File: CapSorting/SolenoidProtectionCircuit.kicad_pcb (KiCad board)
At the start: 2 copper layers, 30 x 30 mm, 15 parts, among them CN12 S6B-XH-A, Q1 2SA1015, Q12 2SA1015, Q13 IRLB8721PBF, Q2 IRLB8721PBF

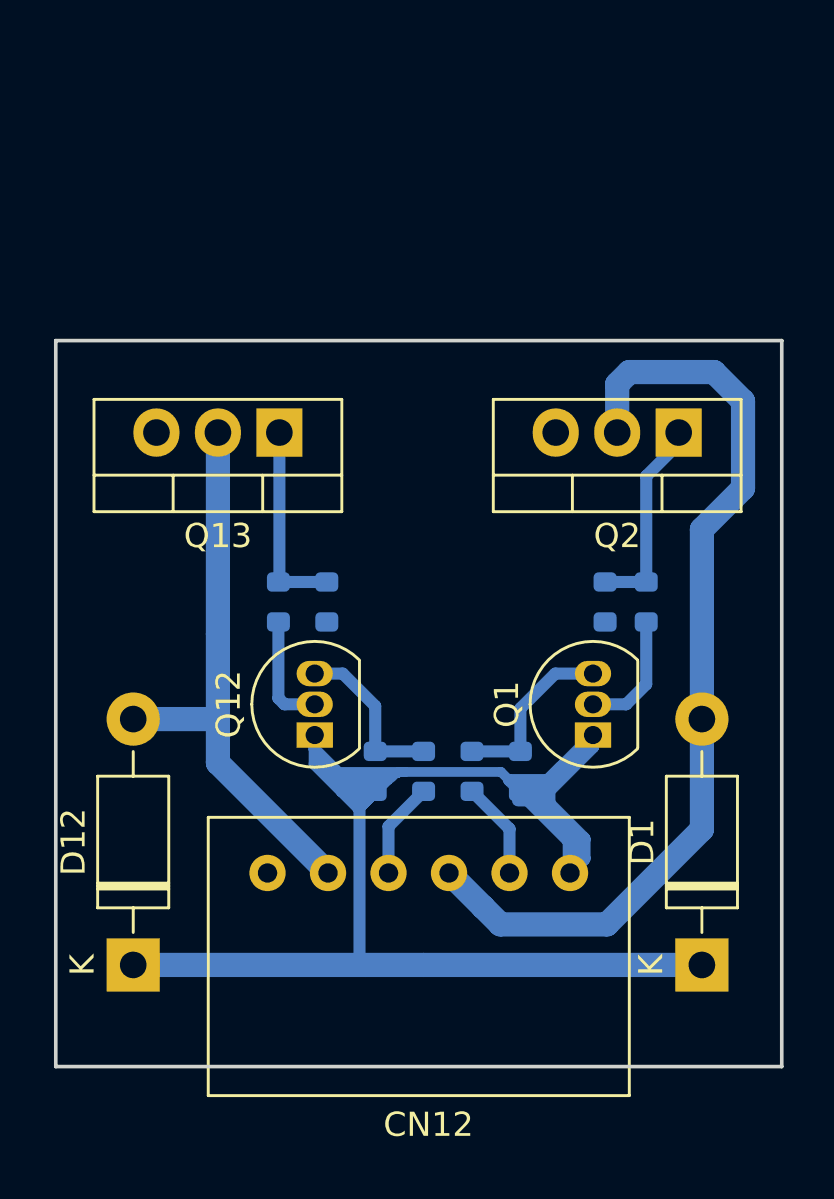
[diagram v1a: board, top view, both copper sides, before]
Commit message: 引き直し
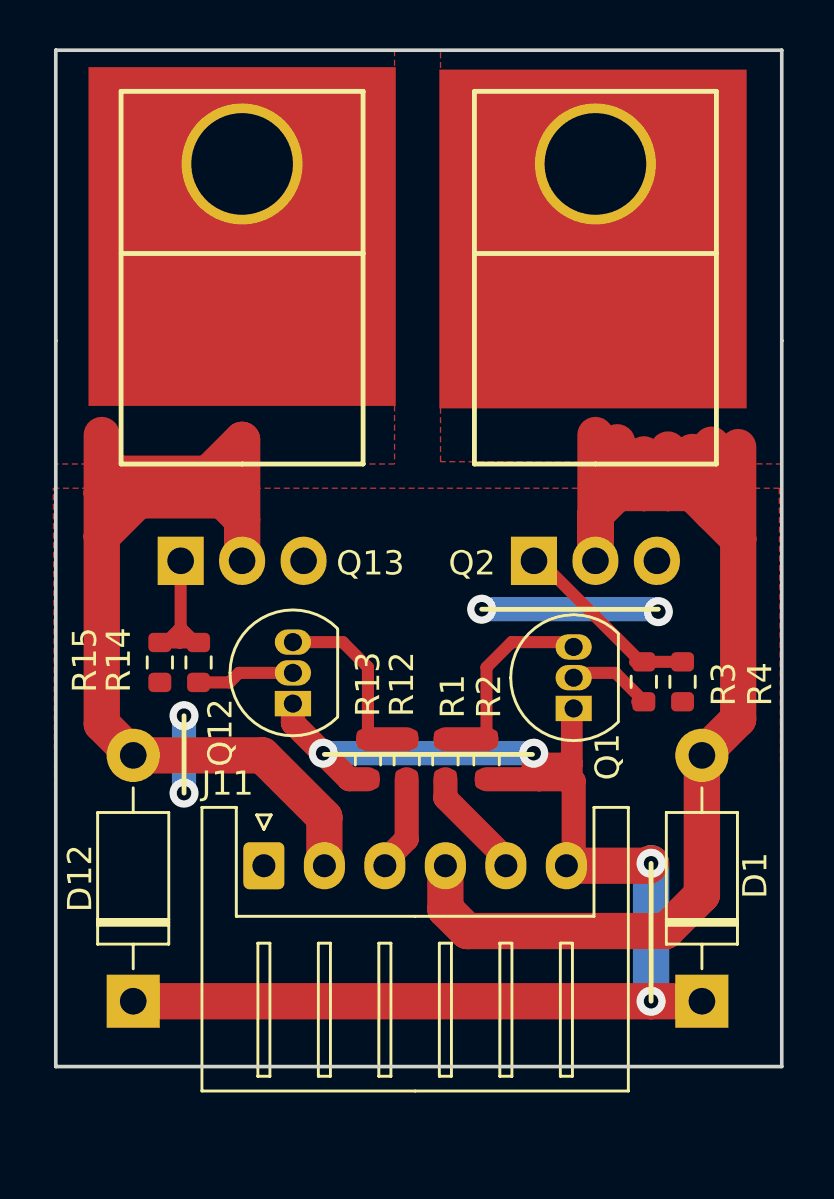
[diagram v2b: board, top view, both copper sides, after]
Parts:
- removed CN12: S6B-XH-A, JST:S6B-XH-A
- added J11: Conn_01x06, Connector_JST:JST_XH_S6B-XH-A_1x06_P2.50mm_Horizontal, F.Cu at (93.6, 99.7)
- Q13, Q2: footprint Package_TO_SOT_THT:TO-220-3_Vertical -> CapSorting:IRLB8721PBF-2
- R1, R12, R13, R14, R15, R2, R3, R4: moved to F.Cu
- moved R15 7.34 mm to (89.3, 91.3)
- moved Q2 6.32 mm to (107.3, 87.1), turned to 0 degrees
- moved Q13 5.52 mm to (92.7, 87.1), turned to 0 degrees
- moved R4 4.60 mm to (110.9, 92.1)
- moved R14 4.14 mm to (90.9, 91.3)
- moved R3 3.30 mm to (109.3, 92.1)
- moved Q12 1.58 mm to (94.8, 93.0)
- moved D1 1.50 mm to (111.7, 105.3)
- moved D12 1.50 mm to (88.2, 105.3)
- moved R2 1.49 mm to (102.8, 95.3)
- moved Q1 1.36 mm to (106.4, 93.2)
- moved R1 1.21 mm to (101.1, 95.3)
- moved R12 0.86 mm to (99.5, 95.3)
- moved R13 0.58 mm to (97.9, 95.3)
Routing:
- net Solenoid1: track 23.6 -> 43.2 mm
- net Solenoid2: track 39.3 -> 56.7 mm
- net +24V: track 74.0 -> 59.4 mm, vias 0 -> 4
- net GND: track 0.00 -> 10.5 mm, vias 0 -> 4
- net Net-(Q1-Pad2): track 5.12 -> 3.68 mm
- net Net-(Q1-Pad3): track 7.37 -> 8.71 mm
- net Net-(Q12-Pad3): track 6.93 -> 8.11 mm
- net Net-(Q13-Pad1): track 8.19 -> 7.10 mm
- net Net-(Q12-Pad2): track 4.76 -> 4.06 mm
- net PLC_Y012: track 4.02 -> 4.61 mm
- added copper zone on F.Cu, net GND
- added copper zone on F.Cu, net Solenoid1
- added copper zone on F.Cu, net Solenoid2
- removed copper zone on B.Cu, net GND
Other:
- board size 30 x 30 mm -> 30 x 42 mm
